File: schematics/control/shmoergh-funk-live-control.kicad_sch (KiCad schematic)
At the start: 5 parts

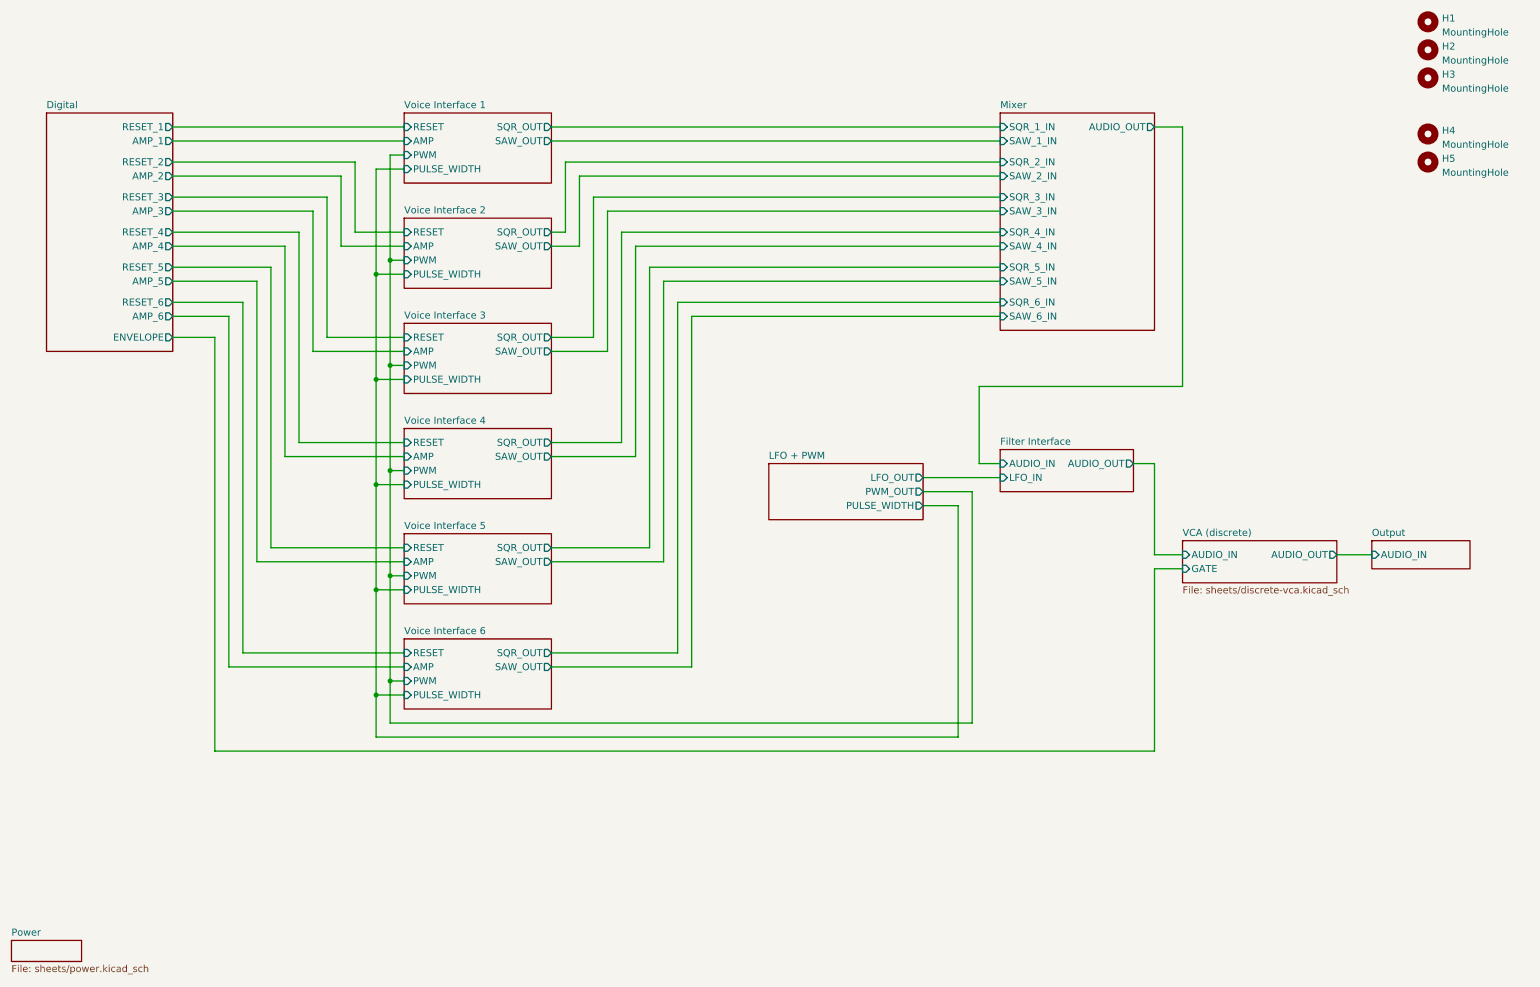
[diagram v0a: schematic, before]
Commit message: Updated VCA
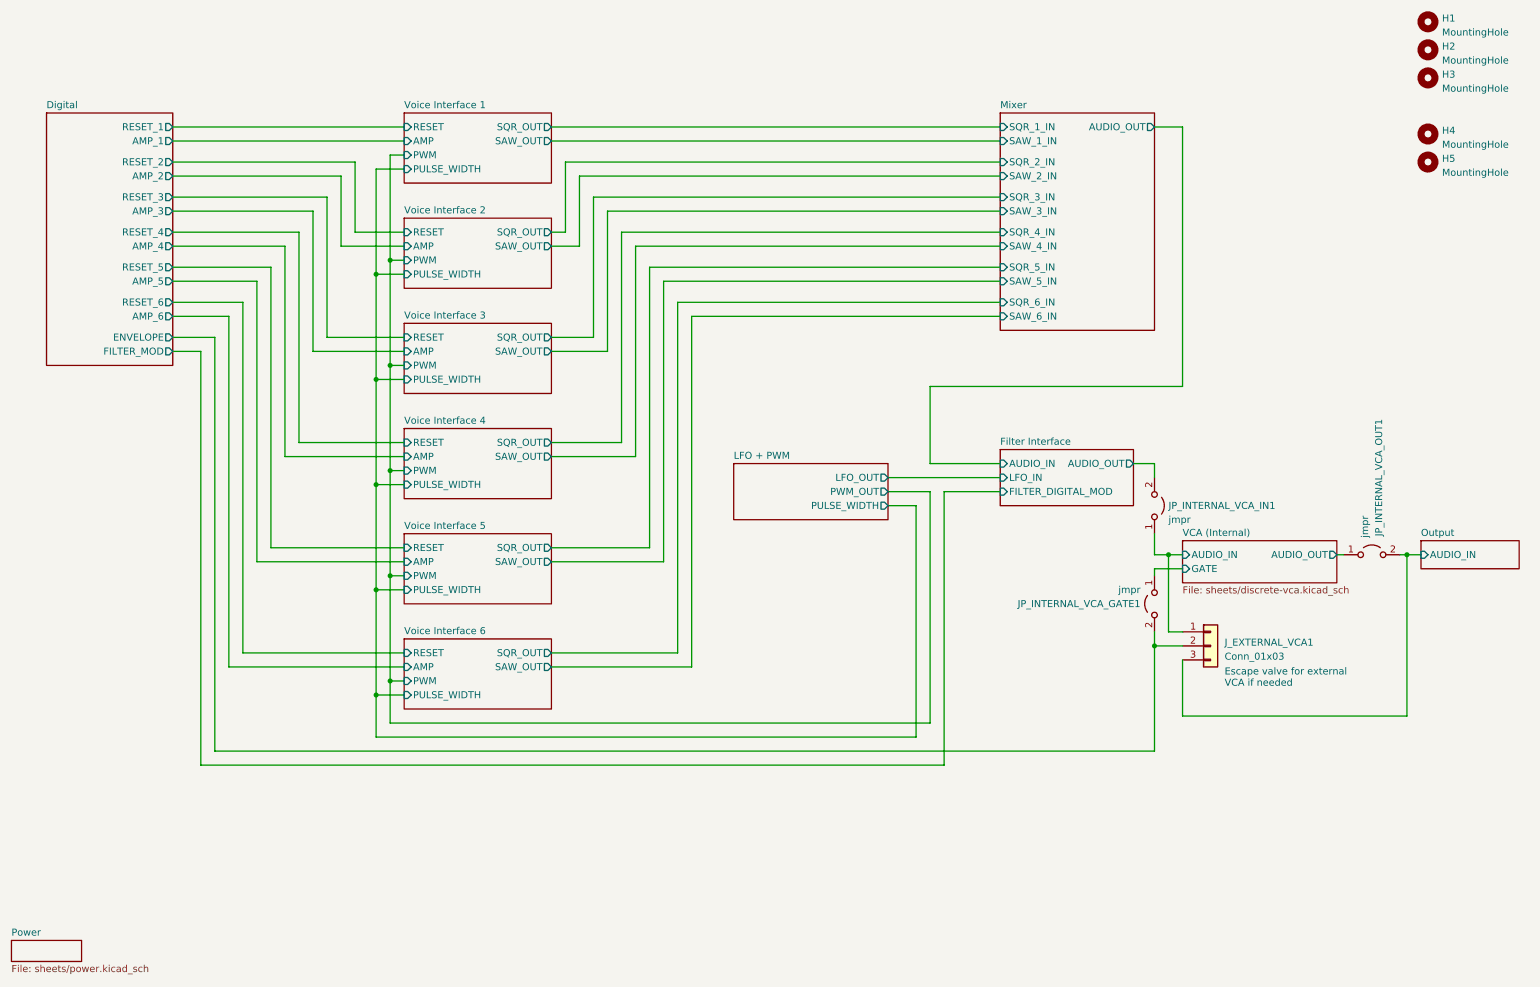
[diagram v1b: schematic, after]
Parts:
- added JP_INTERNAL_VCA_GATE1, JP_INTERNAL_VCA_IN1, JP_INTERNAL_VCA_OUT1: jmpr, symbol Jumper:Jumper_2_Open
- added J_EXTERNAL_VCA1: Conn_01x03, symbol Connector_Generic:Conn_01x03
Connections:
- net Digital/ENVELOPE: now also JP_INTERNAL_VCA_GATE1.2 (B), J_EXTERNAL_VCA1.2 (Pin_2)
- net Filter Interface/AUDIO_OUT: now also JP_INTERNAL_VCA_IN1.2 (B)
- net Output/AUDIO_IN: now also JP_INTERNAL_VCA_OUT1.2 (B), J_EXTERNAL_VCA1.3 (Pin_3)
- new net VCA (Internal)/AUDIO_IN: JP_INTERNAL_VCA_IN1.1 (A), J_EXTERNAL_VCA1.1 (Pin_1)
- new net VCA (Internal)/AUDIO_OUT: JP_INTERNAL_VCA_OUT1.1 (A)
- new net VCA (Internal)/GATE: JP_INTERNAL_VCA_GATE1.1 (A)
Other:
- sheet VCA (discrete) renamed VCA (Internal)
- sheet Digital ports: added FILTER_MOD; removed none
- sheet Filter Interface ports: added FILTER_DIGITAL_MOD; removed none
- note added: "Escape valve for external VCA if needed"
